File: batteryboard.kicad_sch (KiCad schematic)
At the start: 4 parts

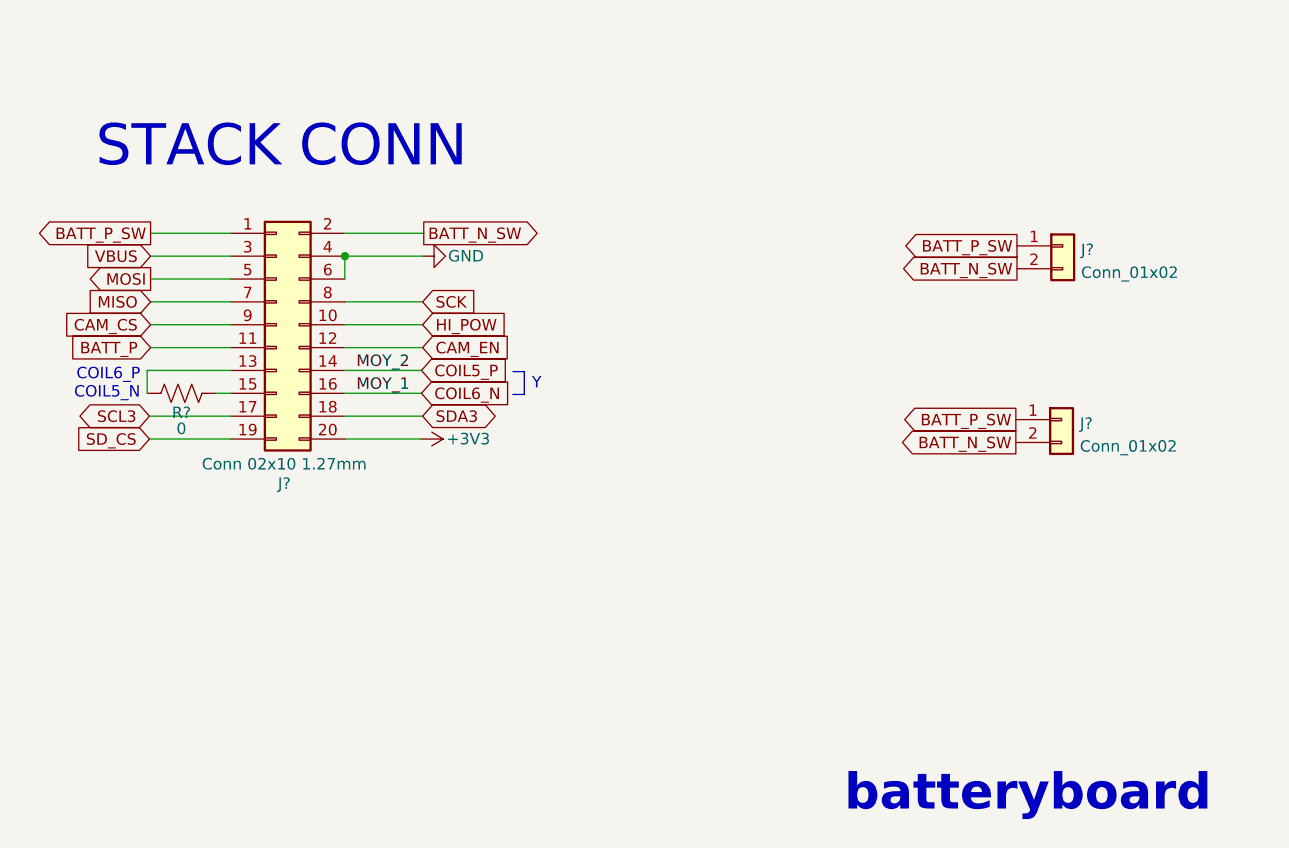
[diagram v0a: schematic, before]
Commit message: completed routing
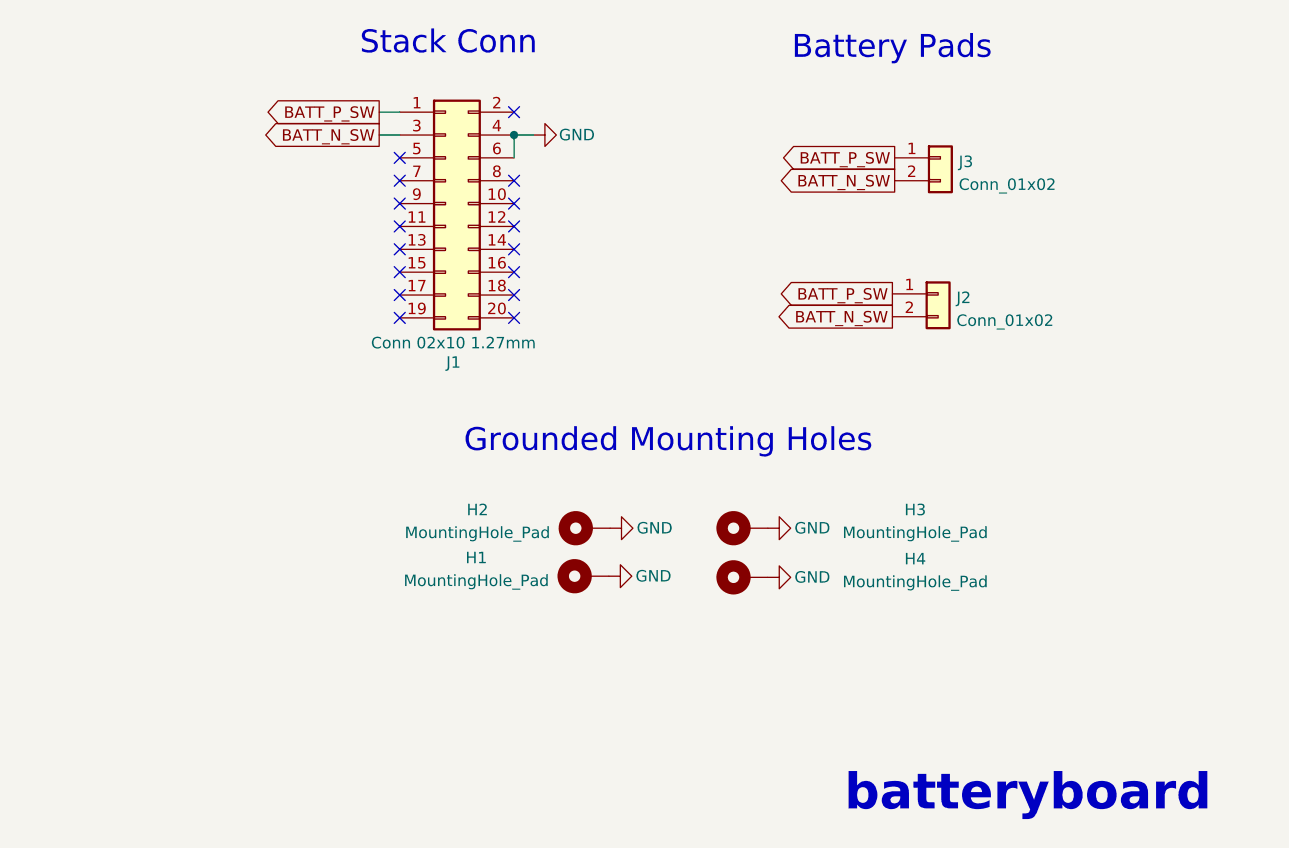
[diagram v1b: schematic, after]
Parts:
- removed R?: 0, Resistor_SMD:R_0603_1608Metric, symbol Device:R_US
- added H1, H2, H3, H4: MountingHole_Pad, mainboard:MountingHole, symbol Mechanical:MountingHole_Pad
- J2, J3: renamed from J?; footprint (none) -> batteryboard:Battery Pads
- gave numbers to parts that had none: 1
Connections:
- net VBUS is gone; now on net BATT_N_SW: J1.3 (Pin_3)
- net BATT_N_SW: no longer J1.2 (Pin_2)
- net GND: now also H1.1, H2.1, H3.1, H4.1
- net +3V3: no longer names the net of J1.20 (Pin_20)
- net BATT_P: no longer names the net of J1.11 (Pin_11)
- net CAM_CS: no longer names the net of J1.9 (Pin_9)
- net CAM_EN: no longer names the net of J1.12 (Pin_12)
- net COIL5_P: no longer names the net of J1.14 (Pin_14)
- net COIL6_N: no longer names the net of J1.16 (Pin_16)
- net HI_POW: no longer names the net of J1.10 (Pin_10)
- net MISO: no longer names the net of J1.7 (Pin_7)
- net MOSI: no longer names the net of J1.5 (Pin_5)
- net SCK: no longer names the net of J1.8 (Pin_8)
- net SCL3: no longer names the net of J1.17 (Pin_17)
- net SDA3: no longer names the net of J1.18 (Pin_18)
- net SD_CS: no longer names the net of J1.19 (Pin_19)
- no-connect marks 0 -> 16
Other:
- note added: "Battery Pads"
- note added: "Grounded Mounting Holes"
- note added: "Stack Conn"
- note removed: "COIL5_N"
- note removed: "COIL6_P"
- note removed: "STACK CONN"
- note removed: "Y"
- moved on the sheet: J1, J2, J3
